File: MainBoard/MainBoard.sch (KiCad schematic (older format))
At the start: 10 parts, among them P0n1 ON, P1 CONN_01X07, P2 CONN_01X04, P3 CONN_01X04, P4 CONN_01X07, P5 BATTERY, U1 4056_CARG

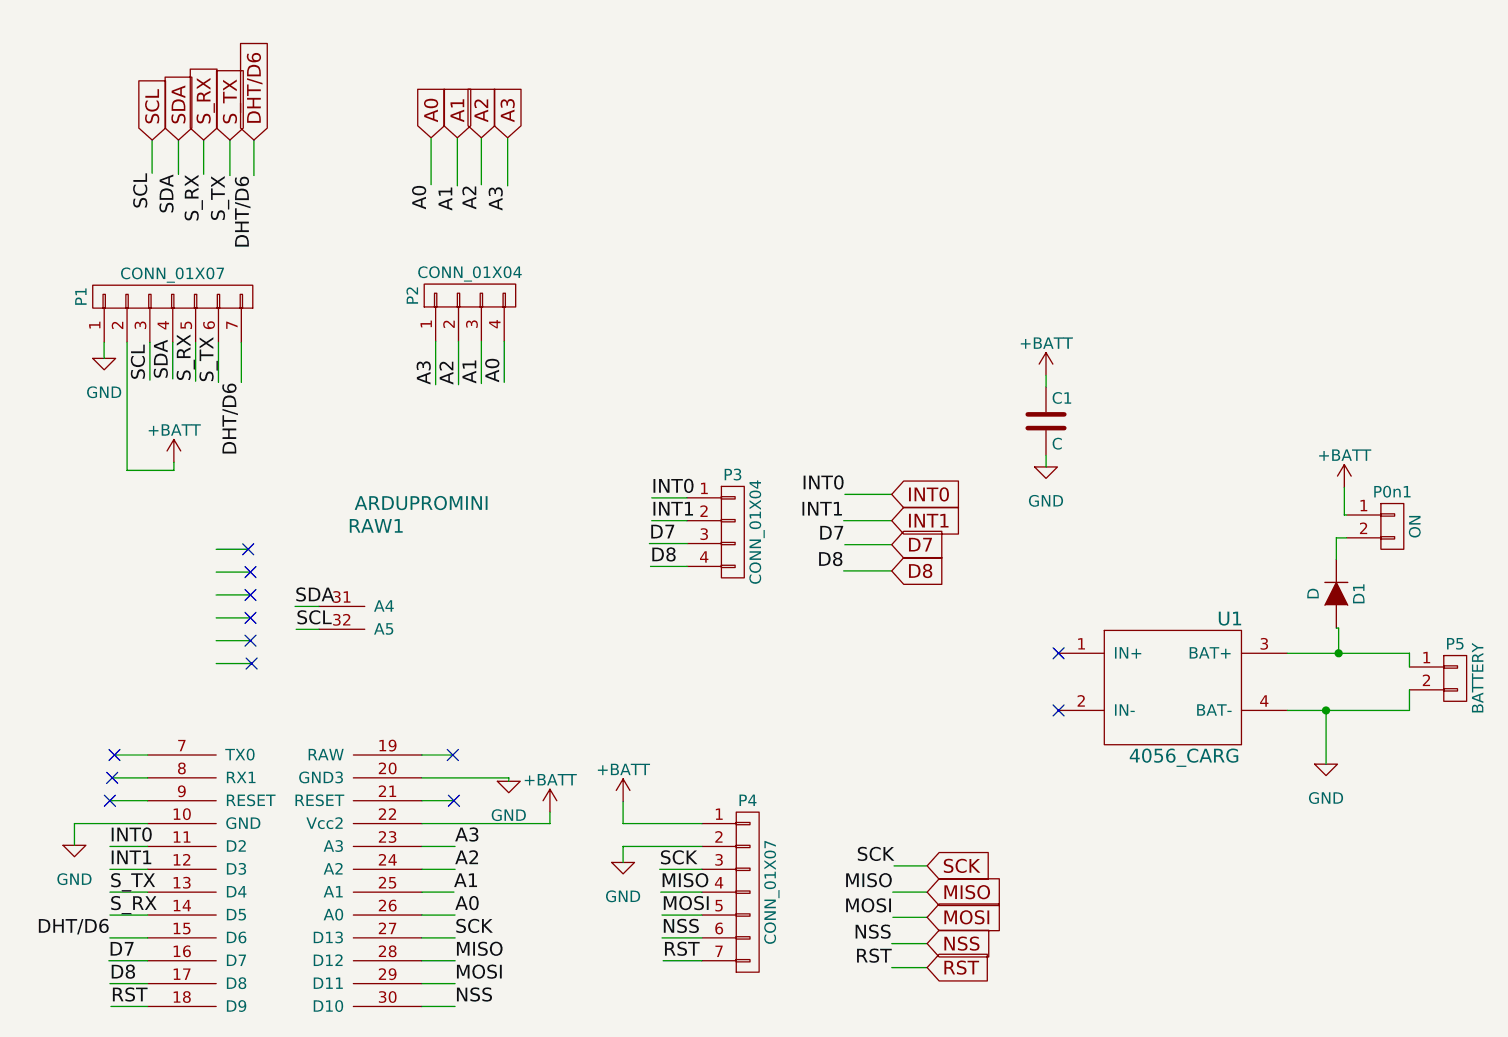
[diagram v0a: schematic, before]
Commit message: Update Schematic MainBoard
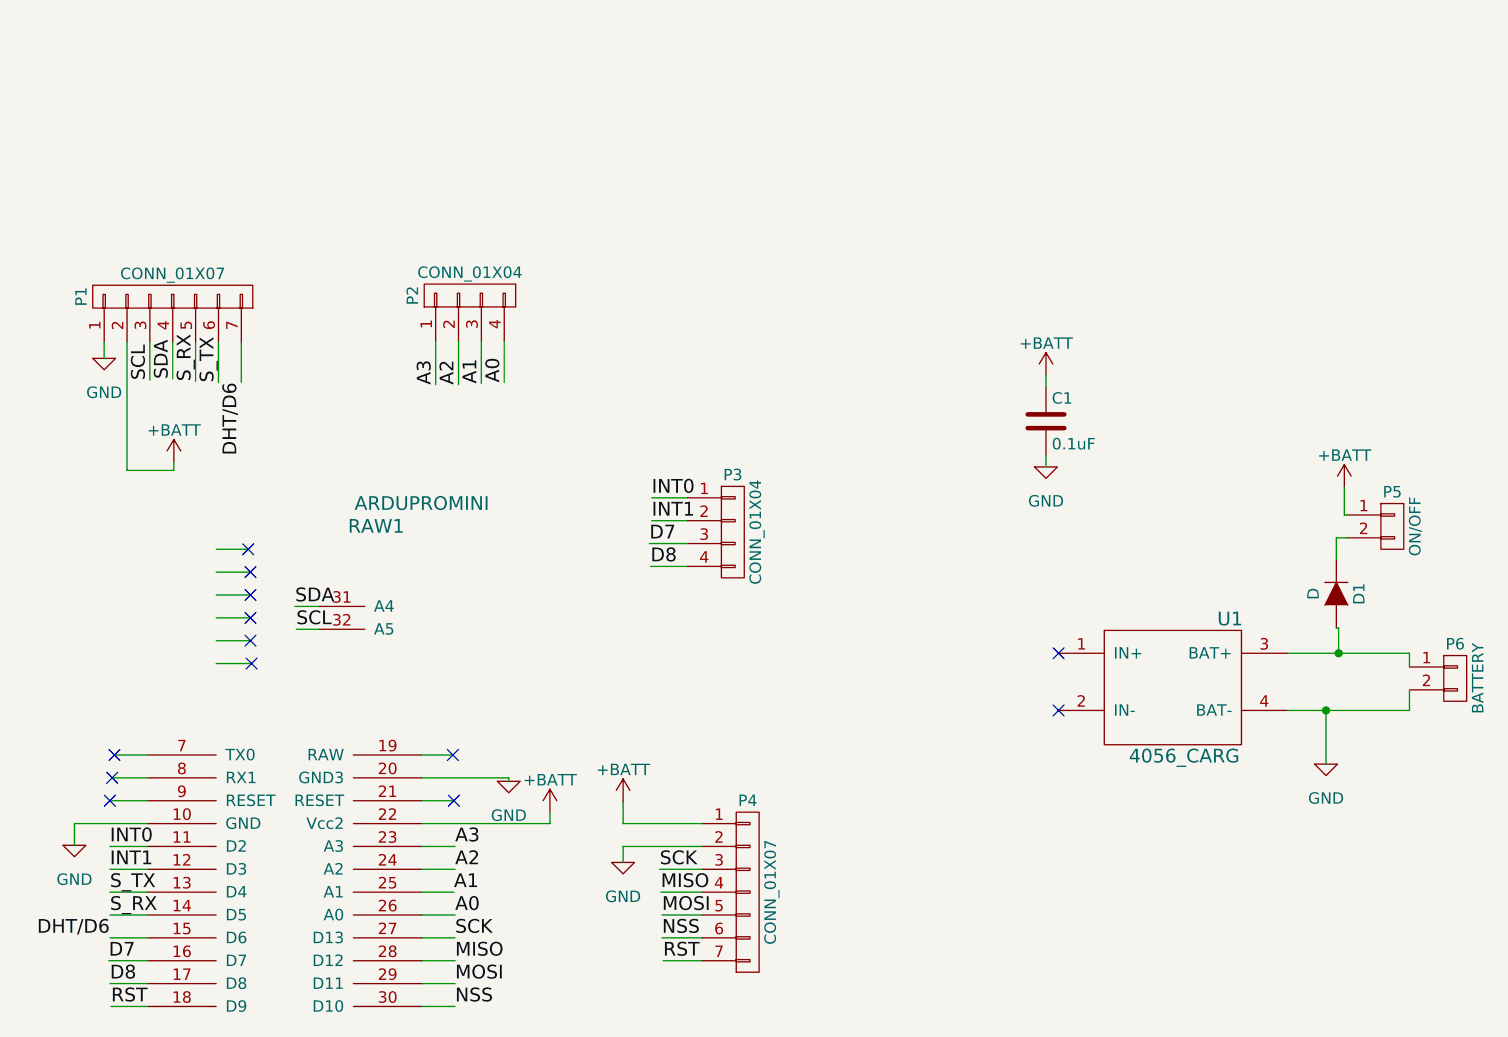
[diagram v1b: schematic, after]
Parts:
- removed P0n1: ON, Pin_Headers:Pin_Header_Straight_1x02, symbol CONN_01X02
- added P5: ON/OFF, Pin_Headers:Pin_Header_Angled_1x02, symbol CONN_01X02
- C1: value C -> 0.1uF
- renumbered P5 to P6
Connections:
- wire segments 93 -> 75
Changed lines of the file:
@@
 EESchema Schematic File Version 2
-LIBS:CatSat-rescue
 LIBS:power
 LIBS:device
@@
 LIBS:contrib
 LIBS:valves
-LIBS:CatSat-cache
+LIBS:MainBoard-cache
 EELAYER 25 0
 EELAYER END
 $Descr A4 11693 8268
 encoding utf-8
-Sheet 2 4
+Sheet 1 1
 Title "CatSat v1.0"
-Date "2016-08-10"
-Rev "0.2"
+Date "2016-10-16"
+Rev "0.3"
 Comp "Electronic Cats"
 Comment1 "Andres Sabas"
@@
 P 4605 4160
 AR Path="/579865C8" Ref="#PWR03"  Part="1"
-AR Path="/57965E31/579865C8" Ref="#PWR03"  Part="1"
+AR Path="/57965E31/579865C8" Ref="#PWR?"  Part="1"
 F 0 "#PWR03" H 4605 3910 50  0001 C CNN
 F 1 "GND" H 4605 4010 50  0000 C CNN
@@
 P 2705 4440
 AR Path="/579869BC" Ref="#PWR04"  Part="1"
-AR Path="/57965E31/579869BC" Ref="#PWR04"  Part="1"
+AR Path="/57965E31/579869BC" Ref="#PWR?"  Part="1"
 F 0 "#PWR04" H 2705 4190 50  0001 C CNN
 F 1 "GND" H 2705 4290 50  0000 C CNN
@@
 $EndComp
 $Comp
-L CONN_01X02 P5
+L CONN_01X02 P6
 U 1 1 57987F4D
 P 8745 3710
-F 0 "P5" H 8745 3860 50  0000 C CNN
+F 0 "P6" H 8745 3860 50  0000 C CNN
 F 1 "BATTERY" V 8845 3710 50  0000 C CNN
 F 2 "Pin_Headers:Pin_Header_Straight_1x02" H 8745 3710 50  0001 C CNN
@@
 P 2835 2310
 AR Path="/5798B584" Ref="#PWR06"  Part="1"
-AR Path="/57965E31/5798B584" Ref="#PWR06"  Part="1"
+AR Path="/57965E31/5798B584" Ref="#PWR?"  Part="1"
 F 0 "#PWR06" H 2835 2060 50  0001 C CNN
 F 1 "GND" H 2835 2160 50  0000 C CNN
@@
 	1    0    0    -1
 $EndComp
-Text GLabel 4600 1345 1    60   Input ~ 0
-A3
-Text GLabel 4485 1345 1    60   Input ~ 0
-A2
-Text GLabel 4380 1345 1    60   Input ~ 0
-A1
-Text GLabel 4265 1345 1    60   Input ~ 0
-A0
-Text GLabel 3160 1355 1    60   Input ~ 0
-SDA
-Text GLabel 3045 1355 1    60   Input ~ 0
-SCL
-Text GLabel 3490 1355 1    60   Input ~ 0
-DHT/D6
-Text GLabel 3385 1355 1    60   Input ~ 0
-S_TX
-Text GLabel 3270 1355 1    60   Input ~ 0
-S_RX
 Wire Wire Line
 	3235 2240 3235 2410
@@
 Wire Wire Line
 	2705 4345 2705 4440
-Wire Wire Line
-	3045 1355 3045 1500
-Wire Wire Line
-	3160 1355 3160 1505
-Wire Wire Line
-	3270 1355 3270 1505
-Wire Wire Line
-	3385 1355 3385 1510
-Wire Wire Line
-	3490 1355 3490 1510
-Wire Wire Line
-	4265 1345 4265 1550
-Wire Wire Line
-	4380 1345 4380 1555
-Wire Wire Line
-	4485 1345 4485 1550
-Wire Wire Line
-	4600 1345 4600 1555
-Text Label 3045 1500 3    60   ~ 0
-SCL
-Text Label 3160 1505 3    60   ~ 0
-SDA
-Text Label 3270 1505 3    60   ~ 0
-S_RX
-Text Label 3385 1510 3    60   ~ 0
-S_TX
-Text Label 3490 1510 3    60   ~ 0
-DHT/D6
-Text Label 4265 1550 3    60   ~ 0
-A0
-Text Label 4380 1555 3    60   ~ 0
-A1
-Text Label 4485 1550 3    60   ~ 0
-A2
-Text Label 4600 1555 3    60   ~ 0
-A3
-Text GLabel 6280 3240 2    60   Input ~ 0
-D8
-Text GLabel 6280 3125 2    60   Input ~ 0
-D7
-Text GLabel 6280 3020 2    60   Input ~ 0
-INT1
-Text GLabel 6280 2905 2    60   Input ~ 0
-INT0
-Text GLabel 6435 4645 2    60   Input ~ 0
-MISO
-Text GLabel 6435 4530 2    60   Input ~ 0
-SCK
-Text GLabel 6435 4975 2    60   Input ~ 0
-RST
-Text GLabel 6435 4870 2    60   Input ~ 0
-NSS
-Text GLabel 6435 4755 2    60   Input ~ 0
-MOSI
-Wire Wire Line
-	6435 4530 6290 4530
-Wire Wire Line
-	6435 4645 6285 4645
-Wire Wire Line
-	6435 4755 6285 4755
-Wire Wire Line
-	6435 4870 6280 4870
-Wire Wire Line
-	6435 4975 6280 4975
-Wire Wire Line
-	6280 2905 6075 2905
-Wire Wire Line
-	6280 3020 6070 3020
-Text Label 6290 4530 2    60   ~ 0
-SCK
-Text Label 6285 4645 2    60   ~ 0
-MISO
-Text Label 6285 4755 2    60   ~ 0
-MOSI
-Text Label 6280 4870 2    60   ~ 0
-NSS
-Text Label 6280 4975 2    60   ~ 0
-RST
-Text Label 6075 2905 2    60   ~ 0
-INT0
-Text Label 6070 3020 2    60   ~ 0
-INT1
 Wire Wire Line
 	5385 3020 5230 3020
@@
 Text Label 5230 3020 0    60   ~ 0
 INT1
-Wire Wire Line
-	6070 3240 6280 3240
-Text Label 6070 3240 2    60   ~ 0
-D8
-Text Label 6075 3125 2    60   ~ 0
-D7
-Wire Wire Line
-	6075 3125 6280 3125
 $Comp
 L GND-RESCUE-CatSat #PWR07
@@
 P 5105 4515
 AR Path="/579A7004" Ref="#PWR07"  Part="1"
-AR Path="/57965E31/579A7004" Ref="#PWR07"  Part="1"
+AR Path="/57965E31/579A7004" Ref="#PWR?"  Part="1"
 F 0 "#PWR07" H 5105 4265 50  0001 C CNN
 F 1 "GND" H 5105 4365 50  0000 C CNN
@@
 P 6955 2585
 F 0 "C1" H 6980 2685 50  0000 L CNN
-F 1 "C" H 6980 2485 50  0000 L CNN
+F 1 "0.1uF" H 6980 2485 50  0000 L CNN
 F 2 "Capacitors_ThroughHole:C_Disc_D6_P5" H 6993 2435 30  0001 C CNN
 F 3 "" H 6955 2585 60  0000 C CNN
@@
 $EndComp
 $Comp
-L GND-RESCUE-CatSat #PWR?
+L GND-RESCUE-CatSat #PWR010
 U 1 1 579BC6D3
 P 6955 2785
-AR Path="/579BC6D3" Ref="#PWR?"  Part="1"
-AR Path="/57965E31/579BC6D3" Ref="#PWR010"  Part="1"
+AR Path="/579BC6D3" Ref="#PWR010"  Part="1"
+AR Path="/57965E31/579BC6D3" Ref="#PWR?"  Part="1"
 F 0 "#PWR010" H 6955 2535 50  0001 C CNN
 F 1 "GND" H 6955 2635 50  0000 C CNN
@@
 Wire Wire Line
 	8010 3600 8545 3600
-$Comp
-L CONN_01X02 P0n1
-U 1 1 57A00135
-P 8470 3045
-F 0 "P0n1" H 8470 3195 50  0000 C CNN
-F 1 "ON" V 8570 3045 50  0000 C CNN
-F 2 "Pin_Headers:Pin_Header_Straight_1x02" H 8470 3045 50  0001 C CNN
-F 3 "" H 8470 3045 50  0000 C CNN
-	1    8470 3045
-	1    0    0    -1
-$EndComp
 Wire Wire Line
 	8260 2995 8270 2995
@@
 	8235 3490 8225 3490
 $Comp
-L GND-RESCUE-CatSat #PWR?
+L GND-RESCUE-CatSat #PWR011
 U 1 1 57AC0CD8
 P 8180 4085
-AR Path="/57AC0CD8" Ref="#PWR?"  Part="1"
+AR Path="/57AC0CD8" Ref="#PWR011"  Part="1"
 AR Path="/57965E31/57AC0CD8" Ref="#PWR?"  Part="1"
-F 0 "#PWR?" H 8180 3835 50  0001 C CNN
+F 0 "#PWR011" H 8180 3835 50  0001 C CNN
 F 1 "GND" H 8180 3935 50  0000 C CNN
 F 2 "" H 8180 4085 50  0000 C CNN
@@
 $Bitmap
 Pos 9650 6940
-Scale 1.000000
+Scale 1,000000
 Data
 89 50 4E 47 0D 0A 1A 0A 00 00 00 0D 49 48 44 52 00 00 01 77 00 00 01 29 08 06 00 00 00 68 44 62
@@
 EndData
 $EndBitmap
+$Comp
+L CONN_01X02 P5
+U 1 1 5803FCFF
+P 8470 3045
+F 0 "P5" H 8470 3195 50  0000 C CNN
+F 1 "ON/OFF" V 8570 3045 50  0000 C CNN
+F 2 "Pin_Headers:Pin_Header_Angled_1x02" H 8470 3045 50  0001 C CNN
+F 3 "" H 8470 3045 50  0000 C CNN
+	1    8470 3045
+	1    0    0    -1
+$EndComp
 $EndSCHEMATC
